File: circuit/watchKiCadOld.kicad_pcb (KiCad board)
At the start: 2 copper layers, 20 parts, among them SW1 Button A, SW2 Button B, U1 LD1117S33TR_SOT223, U2 ATtiny84A-SSU, U3 SN74HC595D, U4 SN74HC595D, U5 KWM-20882CVB, Y1 4MHz

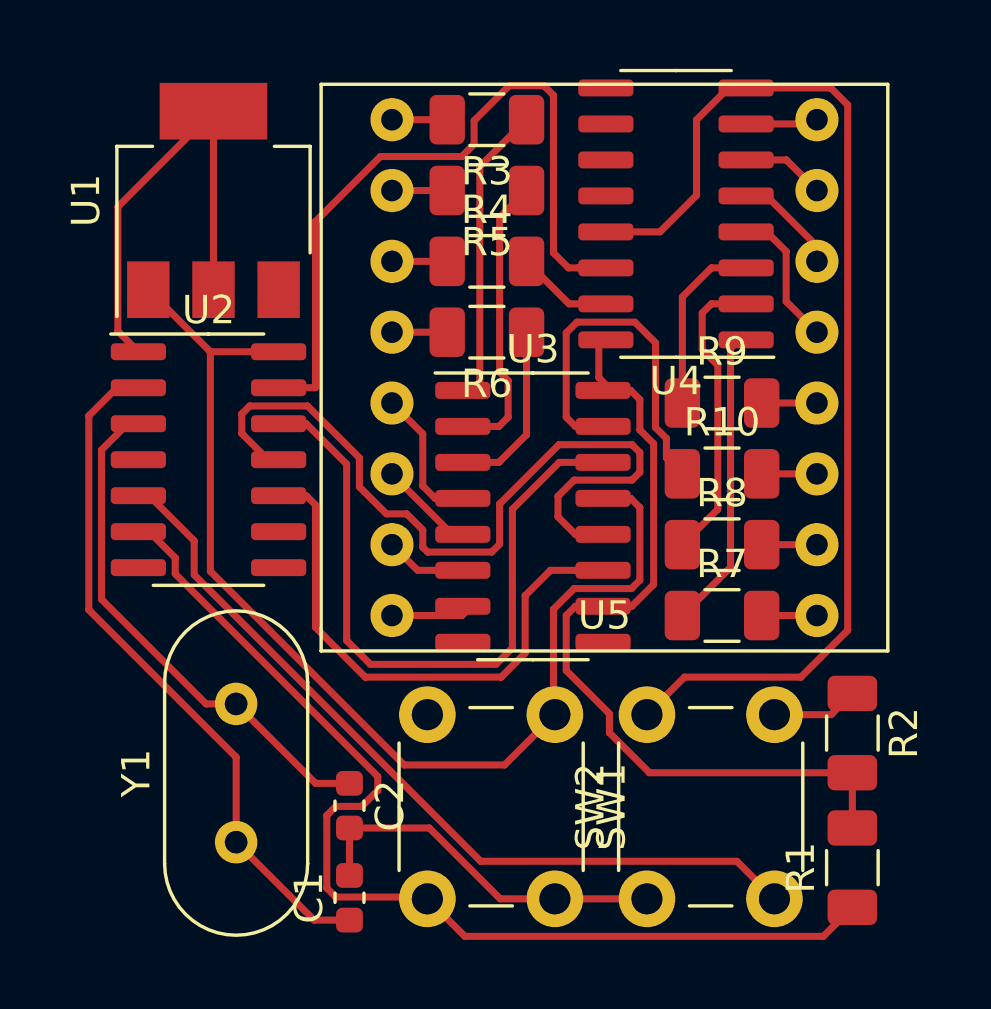
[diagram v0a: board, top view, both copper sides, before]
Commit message: Finished PCB
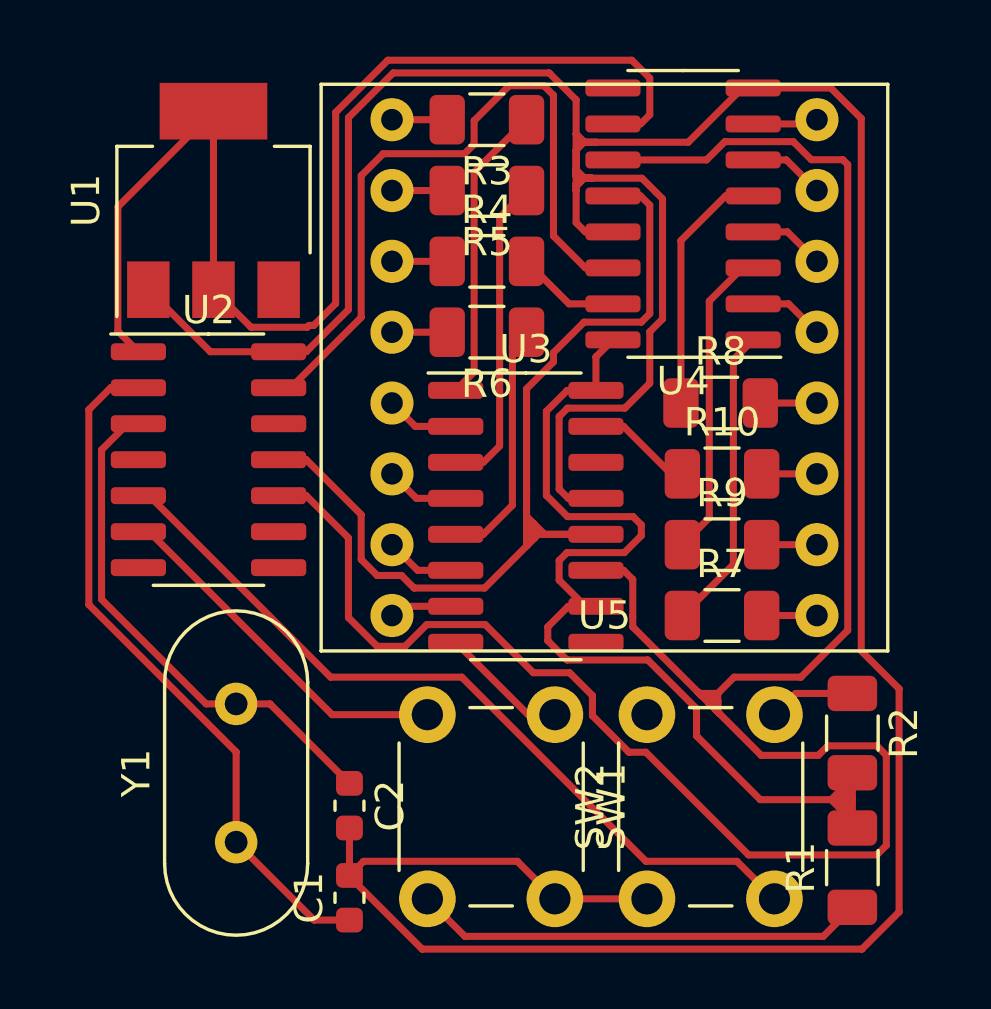
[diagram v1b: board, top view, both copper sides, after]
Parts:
- moved R8 5.00 mm to (164.6, 50.5)
- moved R9 5.00 mm to (164.7, 55.5)
- moved U3 0.25 mm to (157.7, 54.5)
- moved U4 0.25 mm to (163.3, 43.8)
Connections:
- U3 pad 2: Net-(R5-Pad1) -> Net-(U3-Pad2)
- U3 pad 3: Net-(R6-Pad1) -> Net-(R5-Pad1)
- U3 pad 5: Net-(U3-Pad5) -> Net-(R6-Pad1)
- U4 pad 2: Net-(R8-Pad1) -> Net-(U4-Pad2)
- U4 pad 5: Net-(U4-Pad5) -> Net-(R8-Pad1)
- U5 pad 10: Net-(R8-Pad2) -> Net-(R9-Pad2)
- U5 pad 12: Net-(R9-Pad2) -> Net-(R8-Pad2)
- U5 pad 13: Net-(U4-Pad4) -> Net-(U4-Pad2)
- U5 pad 14: Net-(U4-Pad5) -> Net-(U4-Pad4)
- U5 pad 5: Net-(U3-Pad4) -> Net-(U3-Pad2)
- U5 pad 6: Net-(U3-Pad5) -> Net-(U3-Pad4)
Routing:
- net Net-(U2-Pad10): track 20.7 -> 81.4 mm
- net Net-(R1-Pad2): track 46.0 -> 83.9 mm
- net GND: track 93.0 -> 130.6 mm
- net Net-(U2-Pad12): track 24.4 -> 0.00 mm
- net Net-(R10-Pad1): track 13.0 -> 3.74 mm
- net Net-(R1-Pad1): track 37.3 -> 28.8 mm
- net Net-(U2-Pad11): track 29.0 -> 35.6 mm
- net Net-(R9-Pad1): track 6.17 -> 11.0 mm
- net Net-(U4-Pad5): track 4.02 -> 0.00 mm
- net Net-(U3-Pad5): track 3.39 -> 0.00 mm
- net Net-(R6-Pad1): track 5.97 -> 8.74 mm
- net Net-(U3-Pad4): track 5.35 -> 2.61 mm
- net Net-(U4-Pad2): track 0.00 -> 2.66 mm
- net Net-(U3-Pad2): track 0.00 -> 2.59 mm
- net Net-(U4-Pad4): track 5.25 -> 2.68 mm
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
